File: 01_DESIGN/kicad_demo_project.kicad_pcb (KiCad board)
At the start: 2 copper layers, 101 parts, among them J1 Screw_Terminal_01x02, J2 Conn_01x02, J3 USB_B_Micro, J4 Conn_01x08, J5 Conn_01x08, SW1 SW_DPST_x2, SW2 SW_DPST_x2, U1 LM2596S-5, U3 STM32H745ZITx, U4 MTFC32GAZAQDW-AAT, U5 OPA2340, U6 ATMEGA324PA, U7 ISO7721DR, U8 TPS7A4533DCQR, Y1 Crystal_GND24, Y2 Crystal_GND24

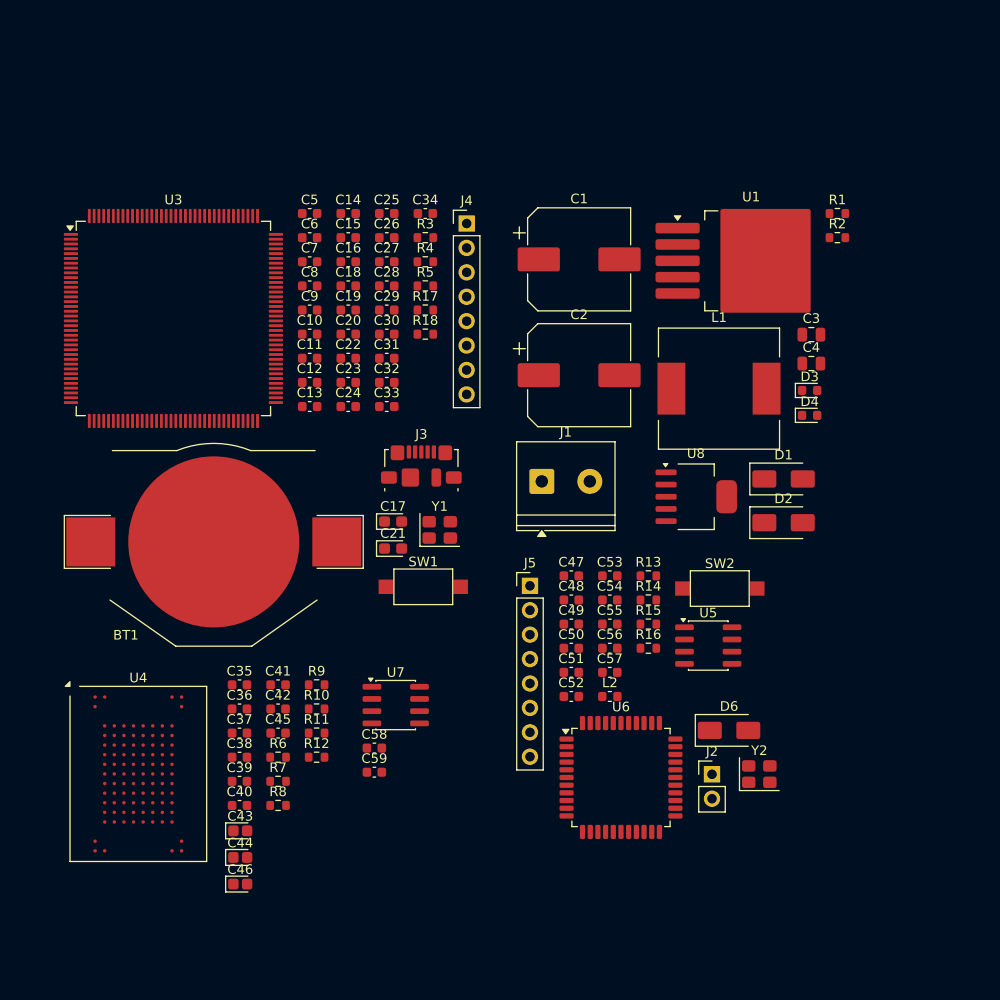
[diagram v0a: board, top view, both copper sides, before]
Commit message: Update project
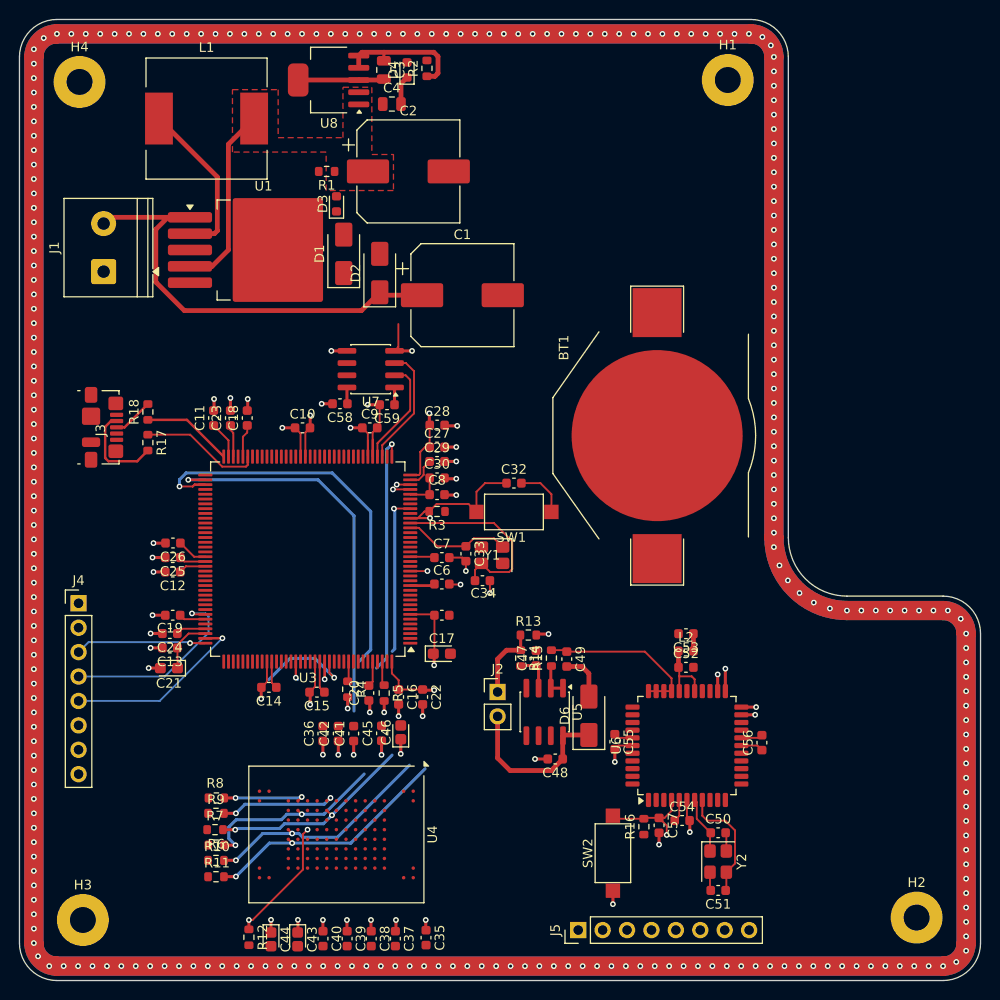
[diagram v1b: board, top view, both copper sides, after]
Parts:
- removed C31: 100nF, Capacitor_SMD:C_0603_1608Metric
- added H1: M3, MountingHole:MountingHole_2.7mm_Pad, F.Cu at (151.9, 58.9)
- added H2: M3, MountingHole:MountingHole_2.7mm_Pad, F.Cu at (171.5, 146.0)
- added H3: M3, MountingHole:MountingHole_2.7mm_Pad, F.Cu at (84.8, 146.3)
- added H4: M3, MountingHole:MountingHole_2.7mm_Pad, F.Cu at (84.4, 59.1)
- D2: value SS24 -> SS34
- L1: value 44uH -> 47uH
- moved L1 60.3 mm to (97.6, 62.9)
- moved U8 57.8 mm to (110.3, 58.9), turned to 180 degrees
- moved J4 56.5 mm to (84.3, 113.3)
- moved D4 55.2 mm to (118.5, 57.8), turned to 90 degrees
- moved R1 53.3 mm to (110.1, 68.4), turned to 180 degrees
- moved D3 52.9 mm to (111.1, 71.8), turned to 90 degrees
- moved C3 52.3 mm to (116.1, 57.8), turned to -90 degrees
- moved D1 51.4 mm to (111.9, 77.0), turned to 90 degrees
- moved C4 51.3 mm to (116.9, 61.4)
- moved U1 50.8 mm to (103.5, 76.6)
- moved J1 50.5 mm to (86.9, 78.8), turned to 90 degrees
- moved C14 50.0 mm to (104.1, 122.1), turned to 180 degrees
- moved D2 49.4 mm to (115.6, 79.0), turned to 90 degrees
- moved BT1 47.4 mm to (144.5, 95.9), turned to -90 degrees
- moved C15 47.4 mm to (109.1, 122.6), turned to 180 degrees
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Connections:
- net Net-(J2-Pin_1) renamed /AVR/NTC1-
- J5 pad 8: /AVR/AVR_JTAG_nRESET -> RESET
- U6 pad 4: unconnected-(U6-~{RESET}-Pad4) -> RESET
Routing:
- net /POWER 12 - 5V & 5 - 3.3V/SHIELDING: track 0.00 -> 1515.2 mm, vias 0 -> 252
- net +3.3V: track 0.00 -> 103.3 mm, vias 0 -> 16
- net GND: track 0.00 -> 103.1 mm, vias 0 -> 38
- net MCU_eMMC_SDMMC2_D1: track 0.00 -> 64.3 mm, vias 0 -> 3
- net MCU_eMMC_SDMMC2_D0: track 0.00 -> 63.0 mm, vias 0 -> 3
- net MCU_eMMC_SDMMC2_CMD: track 0.00 -> 49.7 mm, vias 0 -> 3
- net +12V: track 0.00 -> 48.6 mm
- net +5V: track 0.00 -> 47.0 mm
- net MCU_eMMC_SDMMC2_CK: track 0.00 -> 42.9 mm, vias 0 -> 3
- net /MCU/MCU_JTAG_TCK: track 0.00 -> 21.2 mm, vias 0 -> 1
- net /MCU/MCU_JTAG_TMS: track 0.00 -> 20.4 mm, vias 0 -> 1
- net /MCU/MCU_OSCOUT: track 0.00 -> 20.1 mm
- net MCU_eMMC_SDMMC2_D2: track 0.00 -> 19.1 mm, vias 0 -> 3
- net /AVR/ADC_TEMP1: track 0.00 -> 17.4 mm
- net NRST: track 0.00 -> 17.4 mm, vias 0 -> 1
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- added copper zone on F.Cu, net +5V
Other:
- board outline added: 100 x 100 mm
- copper layers 2 -> 4
